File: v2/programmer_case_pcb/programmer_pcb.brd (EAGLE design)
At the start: 100 x 100 mm, 21 parts, among them J1 1X2-3.5MM

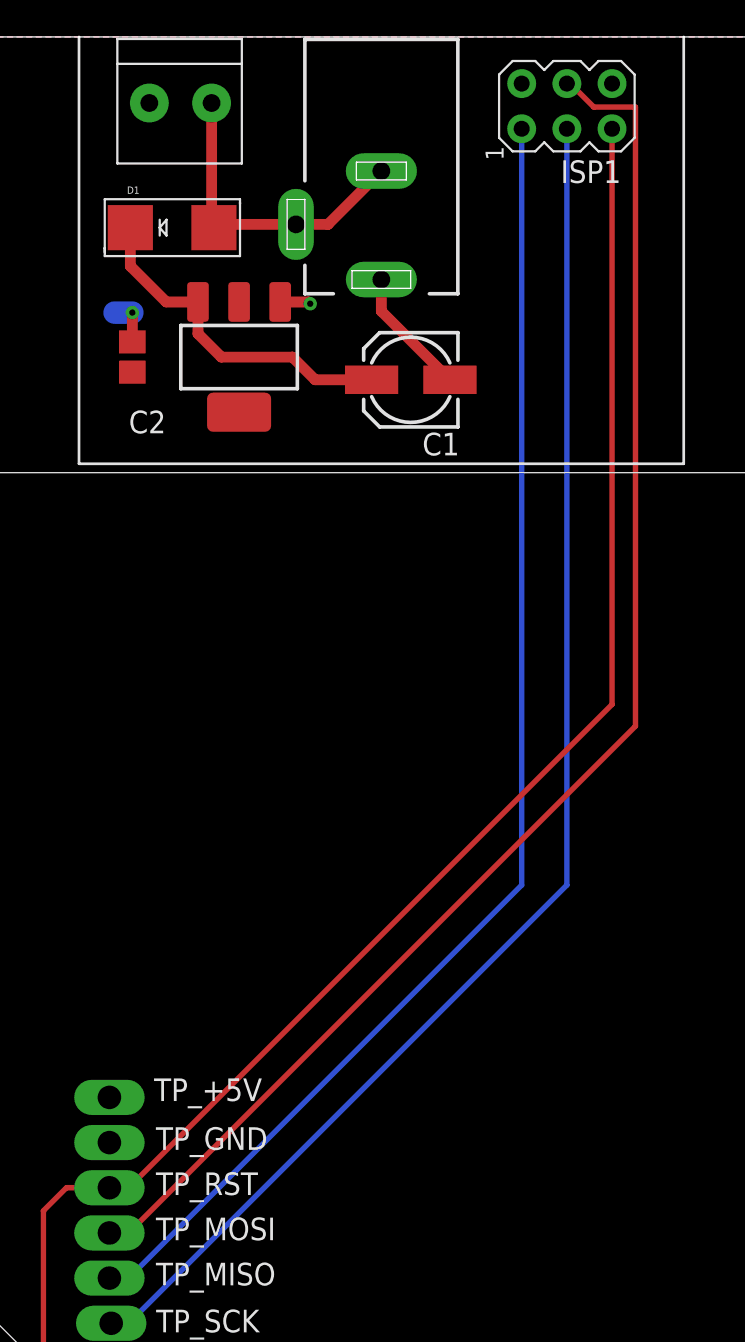
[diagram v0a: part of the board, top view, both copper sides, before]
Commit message: add zip with gerber files
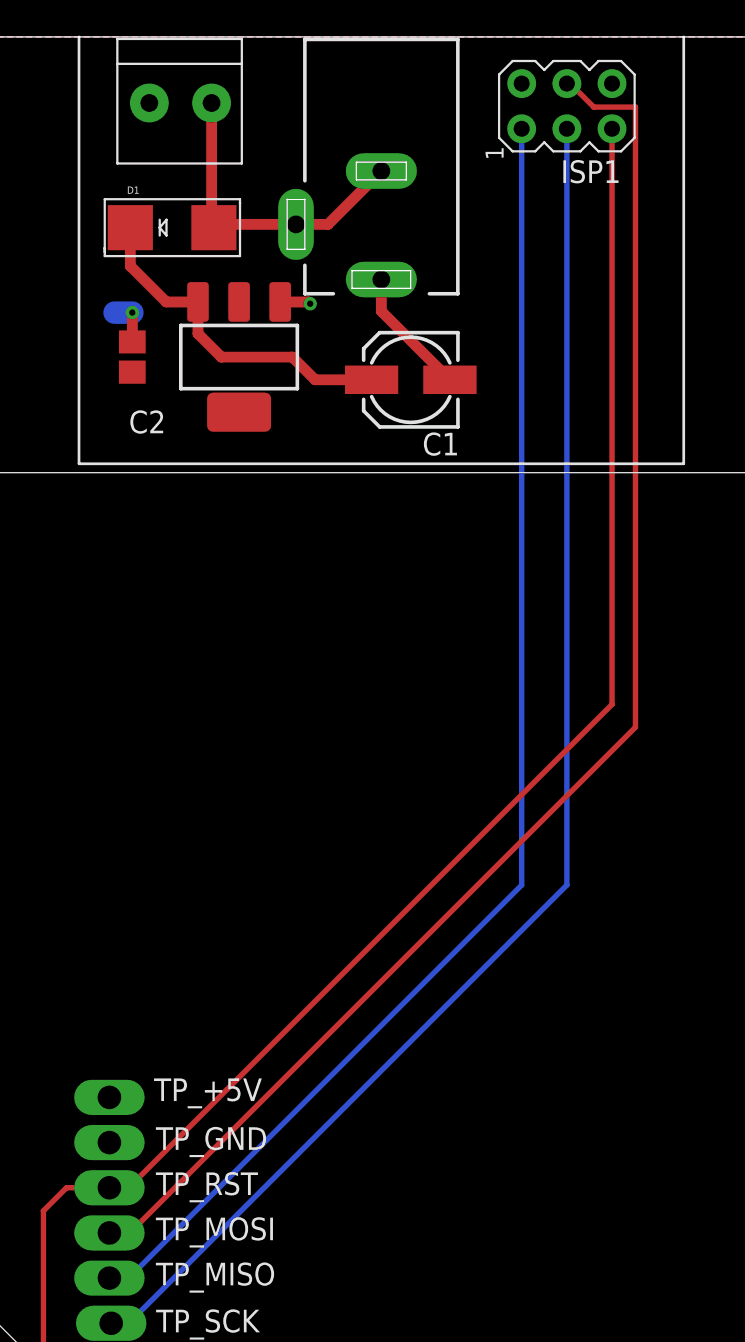
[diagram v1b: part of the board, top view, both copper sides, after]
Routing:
- net MOSI: track 81.6 -> 80.6 mm
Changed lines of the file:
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@@
 <setting verticaltext="up"/>
 </settings>
-<grid distance="0.1" unitdist="mm" unit="mm" style="lines" multiple="1" display="yes" altdistance="5" altunitdist="mil" altunit="mil"/>
+<grid distance="0.01" unitdist="mm" unit="mm" style="lines" multiple="1" display="yes" altdistance="5" altunitdist="mil" altunit="mil"/>
 <layers>
 <layer number="1" name="Top" color="4" fill="1" visible="yes" active="yes"/>
@@
 <contactref element="TP_MOSI" pad="TP"/>
 <contactref element="ISP1" pad="4"/>
-<wire x1="34.71" y1="32.755" x2="35.76435" y2="32.755" width="0.3048" layer="1"/>
-<wire x1="64.2876" y1="61.250025" x2="64.2876" y2="96.0546" width="0.3048" layer="1"/>
-<wire x1="64.2876" y1="96.0546" x2="61.9454" y2="96.0546" width="0.3048" layer="1"/>
+<wire x1="61.9454" y1="96.0546" x2="64.2876" y2="96.0546" width="0.3048" layer="1"/>
 <wire x1="60.623" y1="97.377" x2="60.43" y2="97.377" width="0.3048" layer="1"/>
 <wire x1="61.9454" y1="96.0546" x2="60.623" y2="97.377" width="0.3048" layer="1"/>
-<wire x1="34.71" y1="32.755" x2="35.792575" y2="32.755" width="0.3048" layer="1"/>
-<wire x1="35.792575" y1="32.755" x2="64.2876" y2="61.250025" width="0.3048" layer="1"/>
+<wire x1="64.2876" y1="61.1876" x2="35.85" y2="32.75" width="0.3048" layer="1"/>
+<wire x1="35.85" y1="32.75" x2="34.715" y2="32.75" width="0.3048" layer="1"/>
+<wire x1="34.715" y1="32.75" x2="34.71" y2="32.755" width="0.3048" layer="1"/>
+<wire x1="64.2876" y1="96.0546" x2="64.2876" y2="61.1876" width="0.3048" layer="1"/>
 </signal>
 <signal name="MISO">
